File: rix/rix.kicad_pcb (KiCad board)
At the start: 2 copper layers, 58 x 28 mm, 17 parts, among them J1 Barrel_Jack_Switch, J2 Conn_01x02_Male, J3 Conn_01x01_Male, U1 74LS04, U2 L78L05_SOT89, Y1 Crystal, Y2 Crystal

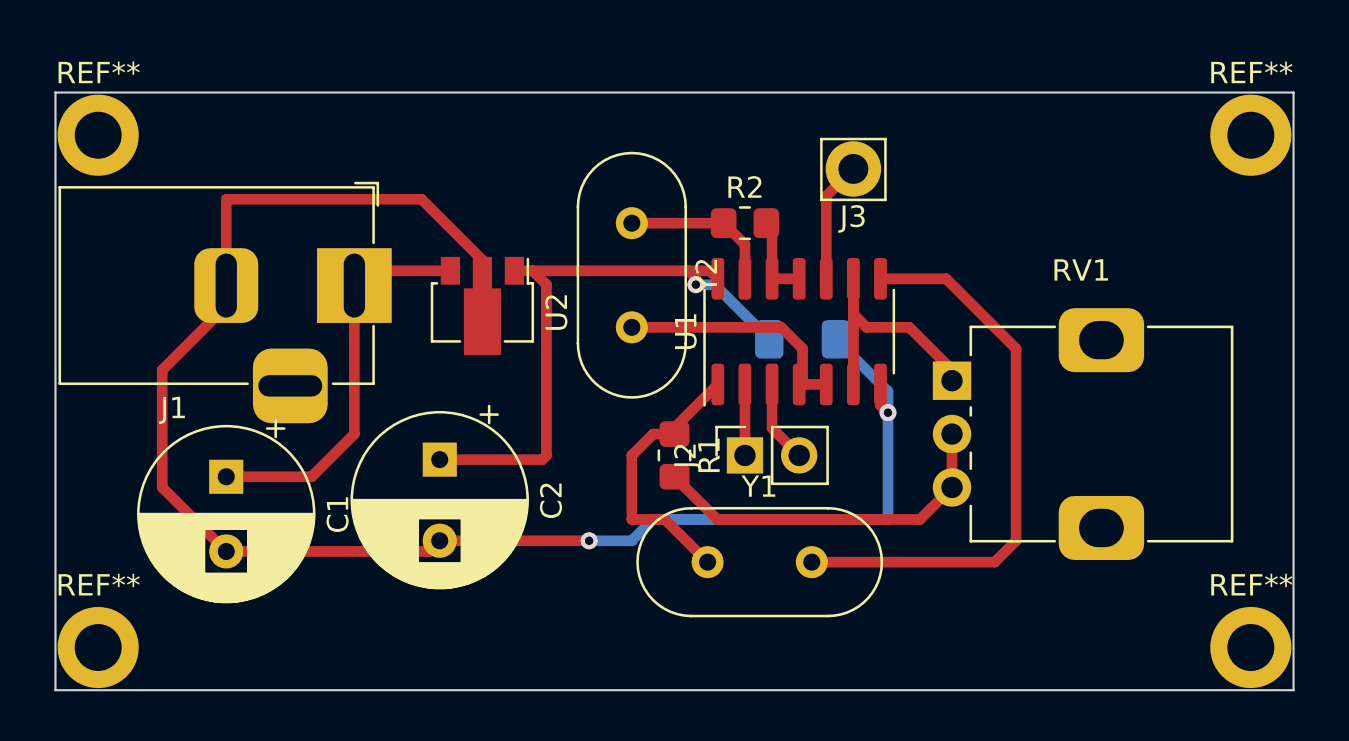
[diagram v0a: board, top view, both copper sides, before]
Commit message: PCB improvements
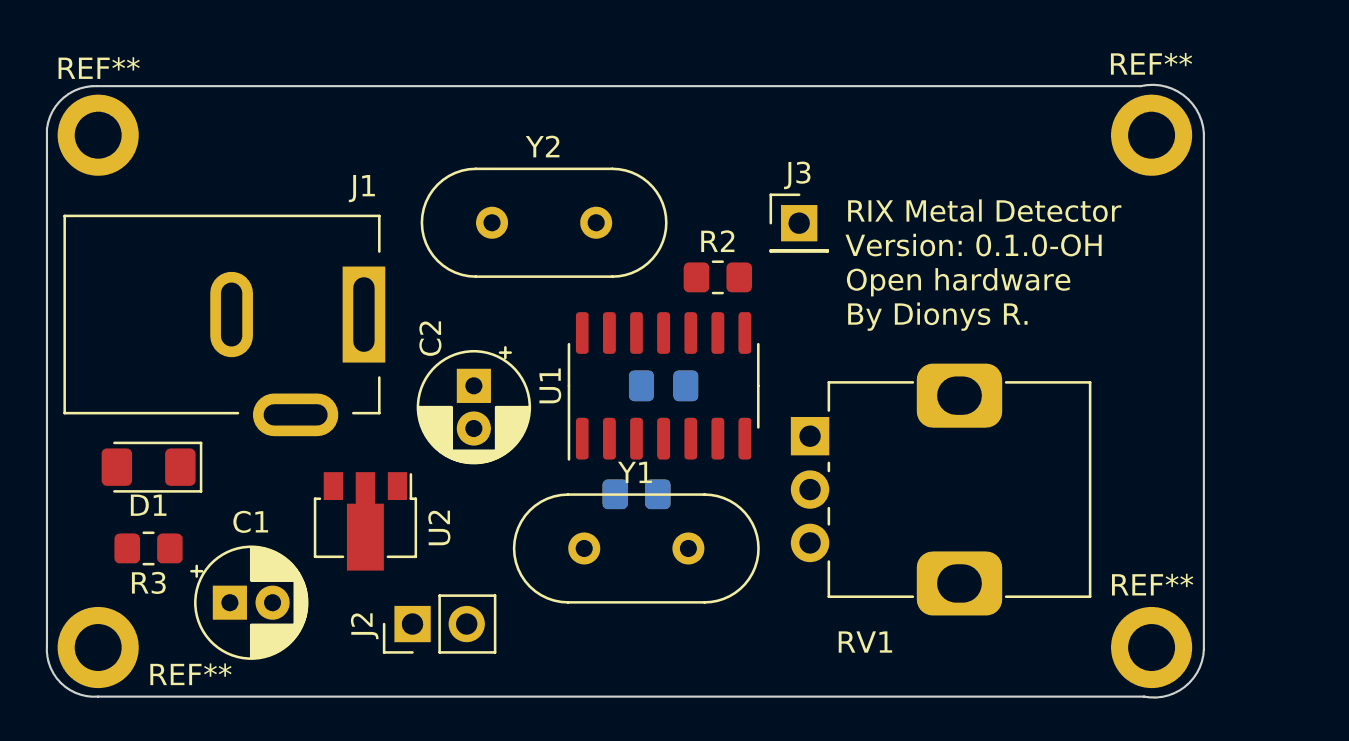
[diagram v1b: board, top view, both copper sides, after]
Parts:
- added D1: LED, Diode_SMD:D_1206_3216Metric_Pad1.42x1.75mm_HandSolder, F.Cu at (86.4, 82.5)
- added R3: 220R, Resistor_SMD:R_0805_2012Metric_Pad1.20x1.40mm_HandSolder, F.Cu at (86.4, 86.4)
- C1: value C_Polarized -> 50v 10uF; footprint Capacitor_THT:CP_Radial_D8.0mm_P3.50mm -> Capacitor_THT:CP_Radial_D5.0mm_P2.00mm
- C2: value C_Polarized -> 50v 1uF; footprint Capacitor_THT:CP_Radial_D8.0mm_P3.80mm -> Capacitor_THT:CP_Radial_D5.0mm_P2.00mm
- C3: value C_Small -> 10nF; footprint Capacitor_SMD:C_1206_3216Metric_Pad1.33x1.80mm_HandSolder -> Capacitor_SMD:C_0805_2012Metric_Pad1.18x1.45mm_HandSolder
- J1: footprint Connector_BarrelJack:BarrelJack_Horizontal -> Connector_BarrelJack:BarrelJack_Kycon_KLDX-0202-xC_Horizontal
- J2: value Conn_01x02_Male -> Detection coil; footprint Connector_PinSocket_2.54mm:PinSocket_1x02_P2.54mm_Vertical -> Connector_PinHeader_2.54mm:PinHeader_1x02_P2.54mm_Vertical
- J3: value Conn_01x01_Male -> External antenna; footprint Connector_Pin:Pin_D1.4mm_L8.5mm_W2.8mm_FlatFork -> Connector_PinHeader_2.54mm:PinHeader_1x01_P2.54mm_Vertical
- R1: value R -> 1M; moved to B.Cu
- RV1: value R_Potentiometer -> 10K
- U1: footprint Package_SO:SO-14_3.9x8.65mm_P1.27mm -> Package_SO:SOIC-14_3.9x8.7mm_P1.27mm
- Y1, Y2: value Crystal -> 8.0 Mhz Crystal
- moved J2 17.5 mm to (98.7, 89.9)
- moved U2 11.5 mm to (96.5, 85.1)
- moved RV1 7.14 mm to (117.3, 81.1)
- moved C3 6.86 mm to (110.5, 78.7)
- moved U1 6.84 mm to (110.5, 78.7)
- moved Y2 6.55 mm to (102.5, 71.1), turned to 0 degrees
- moved C1 5.90 mm to (90.2, 88.9), turned to 0 degrees
- moved Y1 5.82 mm to (106.8, 86.4)
- moved REF** 4.65 mm to (133.3, 91.0)
- moved REF** 4.65 mm to (133.3, 67.0)
- moved C2 3.81 mm to (101.6, 78.7)
- moved J3 3.59 mm to (116.8, 71.1)
- moved R2 2.84 mm to (113.0, 73.7)
- moved R1 2.55 mm to (109.2, 83.8), turned to 0 degrees
- moved J1 1.43 mm to (96.5, 75.4)
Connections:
- J3 pad 1: Net-(U1-Pad10) -> Net-(J3-Pad1)
- R2 pad 1: Net-(U1-Pad13) -> Net-(R2-Pad1)
- R2 pad 2: Net-(U1-Pad12) -> Net-(R2-Pad2)
- U1 pad 10: Net-(U1-Pad10) -> Net-(R2-Pad2)
- U1 pad 11: Net-(U1-Pad12) -> Net-(R2-Pad1)
- U1 pad 13: Net-(U1-Pad13) -> IF
- U1 pad 4: Net-(U1-Pad4) -> IF
- U1 pad 5: Net-(U1-Pad4) -> IF
- U1 pad 8: Net-(U1-Pad8) -> Net-(J3-Pad1)
- U1 pad 9: Net-(RV1-Pad1) -> Net-(R2-Pad2)
- Y1 pad 2: Net-(U1-Pad8) -> Net-(RV1-Pad1)
- Y2 pad 1: Net-(U1-Pad13) -> Net-(U1-Pad12)
- Y2 pad 2: Net-(U1-Pad4) -> Net-(R2-Pad1)
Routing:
- net GND: track 75.5 -> 0.00 mm, vias 2 -> 0
- net Net-(C2-Pad1): track 29.0 -> 0.00 mm, vias 1 -> 0
- net Net-(U1-Pad8): track 26.7 -> 0.00 mm
- net Net-(C1-Pad1): track 18.6 -> 0.00 mm
- net Net-(R1-Pad2): track 16.9 -> 0.00 mm
- net Net-(R1-Pad1): track 13.0 -> 0.00 mm
- net Net-(RV1-Pad1): track 12.8 -> 0.00 mm
- net Net-(U1-Pad4): track 11.4 -> 0.00 mm
- net Net-(U1-Pad13): track 7.32 -> 0.00 mm
- net Net-(U1-Pad10): track 5.67 -> 0.00 mm
- net Net-(U1-Pad12): track 3.99 -> 0.00 mm
- net Net-(J2-Pad2): track 3.85 -> 0.00 mm
- net Net-(J2-Pad1): track 3.33 -> 0.00 mm
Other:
- board size 58 x 28 mm -> 54.2 x 28.7 mm
- board text added: "RIX Metal Detector Version: 0.1.0-OH Open hardware By Dionys R."
